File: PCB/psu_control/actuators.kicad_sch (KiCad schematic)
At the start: 22 parts

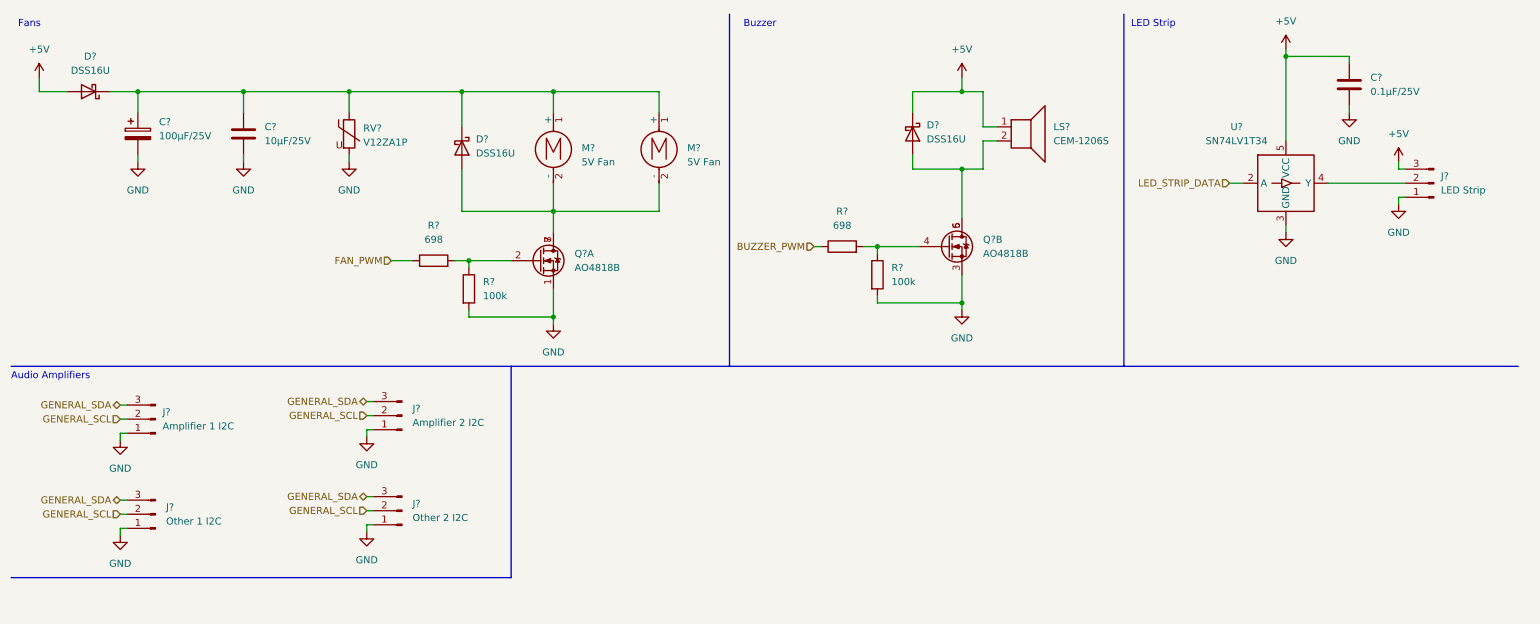
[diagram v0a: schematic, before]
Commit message: psu_control v4 is completed
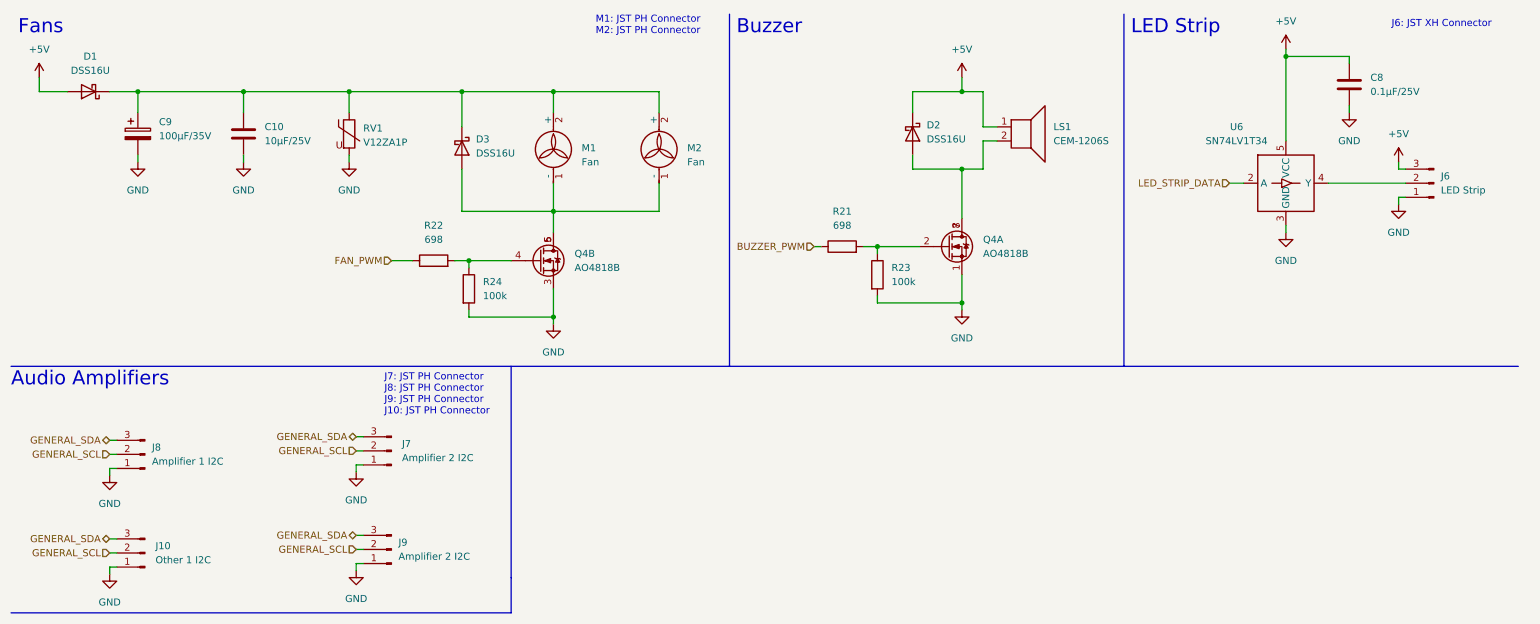
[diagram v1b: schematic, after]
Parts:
- removed J?: Other 2 I2C, symbol Connector:Conn_01x03_Male
- removed M? (x2): 5V Fan, symbol Motor:Motor_DC
- added J9: Amplifier 2 I2C, Connector_JST:JST_PH_B3B-PH-K_1x03_P2.00mm_Vertical, symbol Connector:Conn_01x03_Male
- added M1, M2: Fan, Connector_JST:JST_PH_B2B-PH-K_1x02_P2.00mm_Vertical, symbol t-top:Fan
- C10, C8: renamed from C?; footprint (none) -> Capacitor_SMD:C_0805_2012Metric
- C9: renamed from C?; value 100µF/25V -> 100µF/35V; footprint (none) -> Capacitor_THT:CP_Radial_D6.3mm_P2.50mm
- D1, D2, D3: renamed from D?; footprint (none) -> Diode_SMD:D_SOD-123F
- J10, J7, J8: renamed from J?; footprint (none) -> Connector_JST:JST_PH_B3B-PH-K_1x03_P2.00mm_Vertical
- J6: renamed from J?; footprint (none) -> Connector_JST:JST_XH_B3B-XH-A_1x03_P2.50mm_Vertical
- LS1: renamed from LS?; footprint (none) -> t-top:WT-1205
- Q4: renamed from Q?; footprint (none) -> Package_SO:SOIC-8_3.9x4.9mm_P1.27mm
- R21, R22, R23, R24: renamed from R?; footprint (none) -> Resistor_SMD:R_0805_2012Metric
- RV1: renamed from RV?; footprint (none) -> Varistor:RV_Disc_D7mm_W4mm_P5mm
- gave numbers to parts that had none: 1
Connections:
- net GENERAL_SCL: now also J9.2 (Pin_2)
- net GENERAL_SDA: now also J9.3 (Pin_3)
- net GND: now also Q4.1 (S), Q4.3 (S), J9.1 (Pin_1); no longer Q4.1 (S), Q4.3 (S)
- net at D2.2 (A), LS1.2: now also Q4.7 (D), Q4.8 (D); no longer Q4.5 (D), Q4.6 (D)
- net at C10.1, C9.1, D1.1 (K)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: now also M1.2 (+), M2.2 (+)
- net at R21.2, R23.1: now also Q4.2 (G); no longer Q4.4 (G)
- net at R22.2, R24.1: now also Q4.4 (G); no longer Q4.2 (G)
- new net: D3.2 (A), M1.1 (-), M2.1 (-), Q4.5 (D), Q4.6 (D)
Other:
- note added: "J6: JST XH Connector"
- note added: "J7: JST PH Connector J8: JST PH Connector J9: JST PH Connector J10: JST PH Connector"
- note added: "M1: JST PH Connector M2: JST PH Connector"
- moved on the sheet: J10, J7, J8
